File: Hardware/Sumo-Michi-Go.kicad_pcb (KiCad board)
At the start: 2 copper layers, 87.6 x 69.6 mm, 17 parts, among them J1 ENTRADA, J10 ENTRADA, J11 Conn_01x10, J2 Conn_01x04, J3 Conn_01x09_Pin, J4 SENSOR_INFRAROJO_1, J5 ULTRASONIDO_1, J6 ULTRASONIDO_2, J7 SENSOR_INFRAROJO_2, J8 SENSOR_INFRAROJO_3, J9 ENTRADA, SW1 SWITCH_ON_OFF, SW2 SW_DE_INICIO_ROBOT

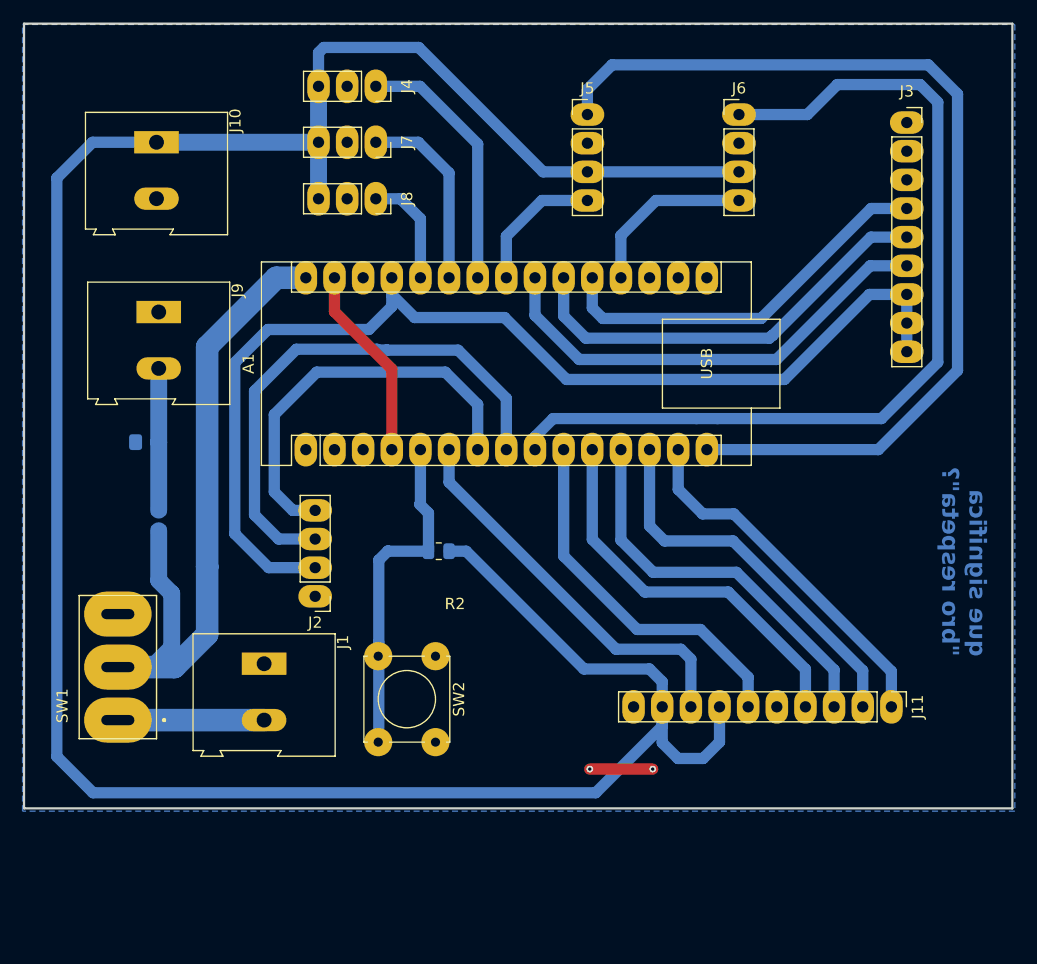
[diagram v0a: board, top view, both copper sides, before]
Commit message: PCB nuevo
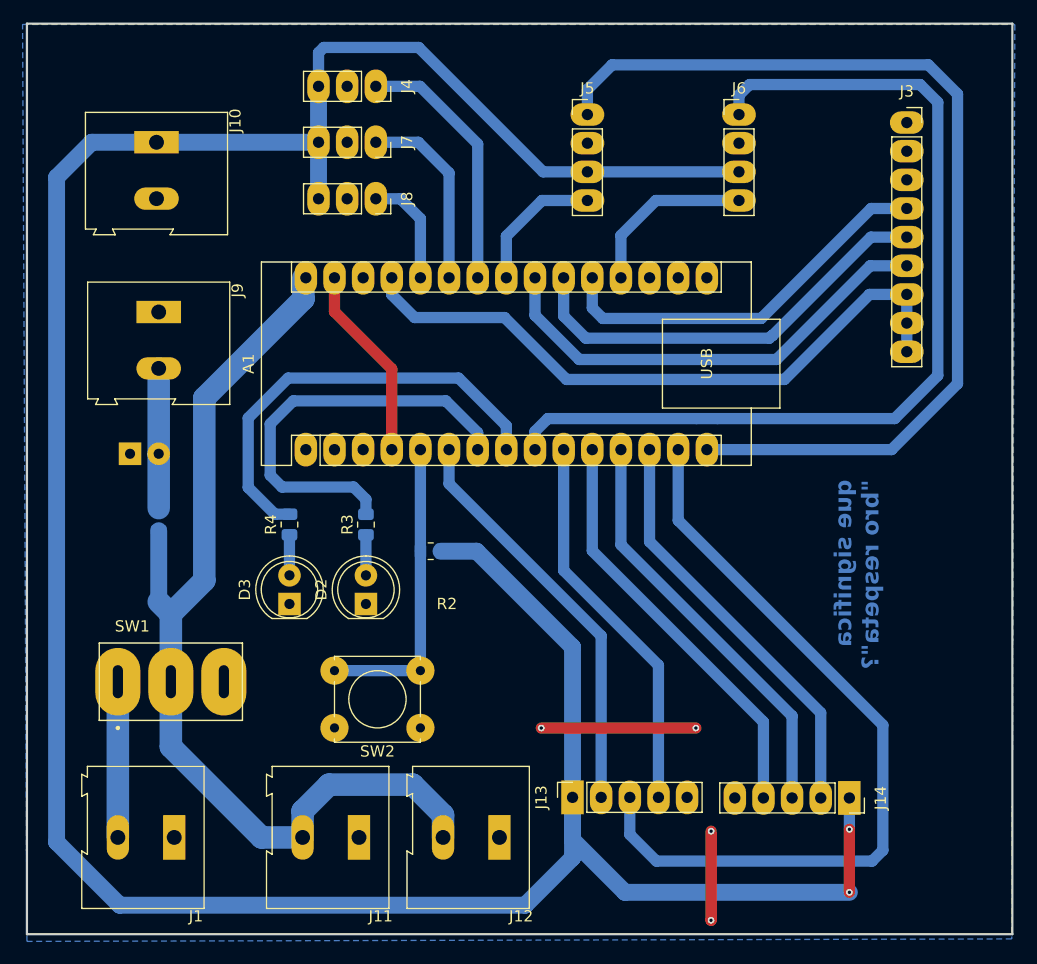
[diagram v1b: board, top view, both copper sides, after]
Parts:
- removed J2: Conn_01x04, Connector_PinHeader_2.54mm:PinHeader_1x04_P2.54mm_Vertical
- added D2: LED, LED_THT:LED_D5.0mm_Clear, F.Cu at (42.6, 67.1)
- added D3: LED, LED_THT:LED_D5.0mm_Clear, F.Cu at (35.9, 67.1)
- added J12: PUENTEH_B, TerminalBlock:TerminalBlock_Altech_AK300-2_P5.00mm, F.Cu at (54.5, 87.8)
- added J13: PUENTEH_A, Connector_PinSocket_2.54mm:PinSocket_1x05_P2.54mm_Vertical, F.Cu at (61.0, 84.2)
- added J14: PUENTEH_B, Connector_PinSocket_2.54mm:PinSocket_1x05_P2.54mm_Vertical, F.Cu at (85.5, 84.3)
- added R3: R, Resistor_SMD:R_0805_2012Metric, F.Cu at (42.6, 60.0)
- added R4: R, Resistor_SMD:R_0805_2012Metric, F.Cu at (35.9, 60.0)
- D1: footprint Inductor_SMD:L_0805_2012Metric_Pad1.15x1.40mm_HandSolder -> LED_THT:LED_D5.0mm_Clear
- J11: value Conn_01x10 -> PUENTEH_A; footprint Connector_PinHeader_2.54mm:PinHeader_1x10_P2.54mm_Vertical -> TerminalBlock:TerminalBlock_Altech_AK300-2_P5.00mm
- J3: value Conn_01x09_Pin -> Sensores_de_piso
- moved J11 48.6 mm to (42.0, 87.8), turned to 180 degrees
- moved J1 17.3 mm to (25.6, 87.8), turned to 180 degrees
- moved SW2 6.50 mm to (47.5, 78.1), turned to 180 degrees
- moved SW1 4.88 mm to (25.3, 74.0), turned to 0 degrees
- moved D1 1.83 mm to (21.7, 53.8)
- moved R2 0.71 mm to (48.4, 62.4)
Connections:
- net Net-(A1-D2) renamed SW_DE_INICIO
- A1 pad 10: ENABLE 2 -> ENABLE_A
- A1 pad 11: ENABLE 1 -> ENABLE_B
- A1 pad 12: PWM 4 -> PWM2_B
- A1 pad 13: PWM 3 -> PWM1_B
- A1 pad 14: PWM 1 -> PWM2_A
- A1 pad 6: PWM2 -> PWM1_A
- A1 pad 7: display -> LED_A
- A1 pad 8: display 2 -> LED_B
- J11 pad 1: PWM 1 -> GND
- J11 pad 2: PWM 3 -> VCC
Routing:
- net PWM2_A: track 0.00 -> 70.2 mm
- net display 2: track 47.5 -> 0.00 mm
- net 5v_arduino: track 100.6 -> 58.5 mm
- net LED_B: track 0.00 -> 39.0 mm
- net PWM2_B: track 0.00 -> 37.2 mm
- net PWM1_B: track 0.00 -> 37.2 mm
- net ENABLE_B: track 0.00 -> 37.2 mm
- net LED_A: track 0.00 -> 37.2 mm
- net PWM1_A: track 0.00 -> 36.4 mm
- net display: track 36.0 -> 0.00 mm
- net PWM2: track 35.1 -> 0.00 mm
- net PWM 4: track 35.0 -> 0.00 mm
- net ENABLE 1: track 35.0 -> 0.00 mm
- net ENABLE_A: track 0.00 -> 34.3 mm
- net PWM 3: track 34.2 -> 0.00 mm
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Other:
- board size 87.6 x 69.6 mm -> 87.4 x 80.7 mm
